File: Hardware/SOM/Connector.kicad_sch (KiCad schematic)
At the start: 1 part, among them J1 SODIMM-200_Split

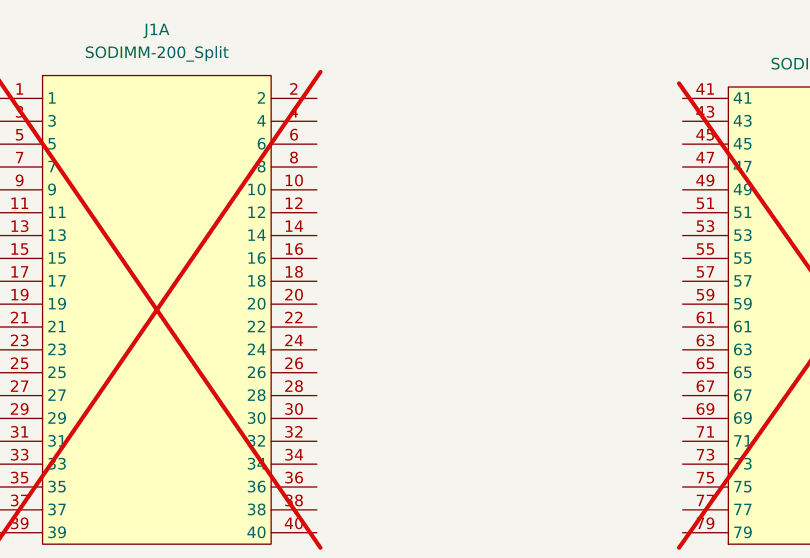
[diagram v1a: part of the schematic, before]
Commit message: SOM: layout update
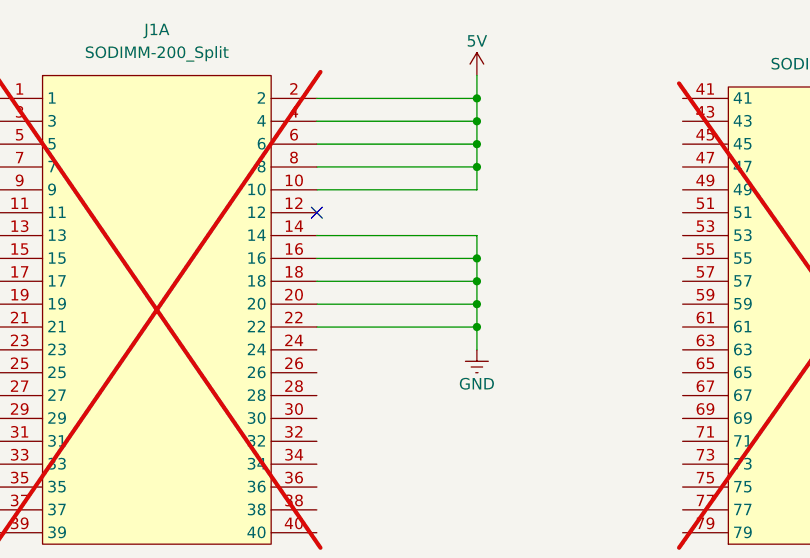
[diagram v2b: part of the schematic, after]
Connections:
- net 5V: now also J1.10, J1.2, J1.4, J1.6, J1.8
- net GND: now also J1.14, J1.16, J1.18, J1.20, J1.22
- no-connect marks 0 -> 1
